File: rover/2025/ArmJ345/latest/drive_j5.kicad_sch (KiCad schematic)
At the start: 13 parts, among them J1 JST_PH_SB6, U1 IFX9201SGAUMA1, U2 CURR_SENSE-INA219AIDCNTG4

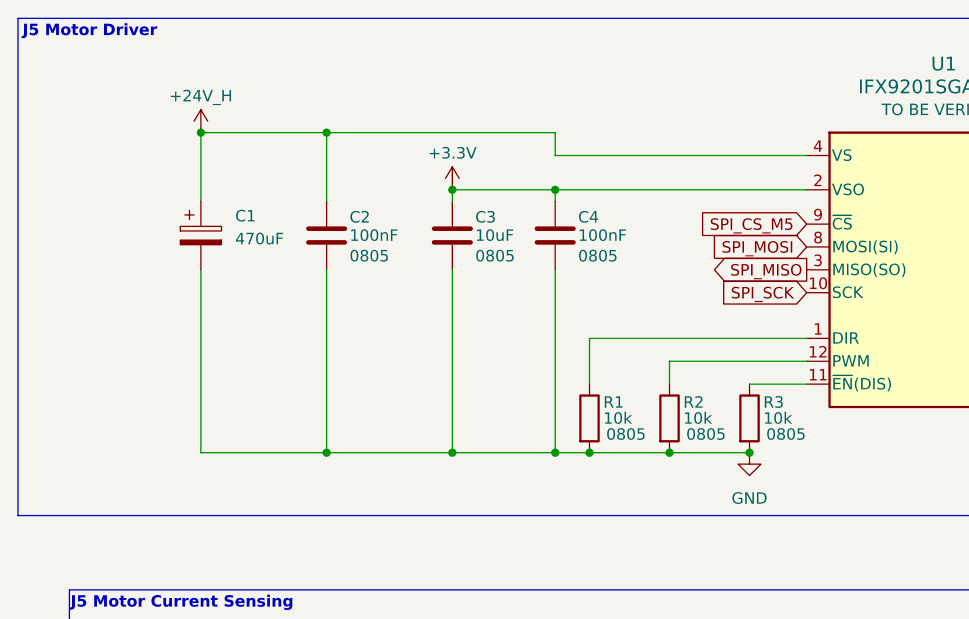
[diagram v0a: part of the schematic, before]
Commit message: armj345 fixes
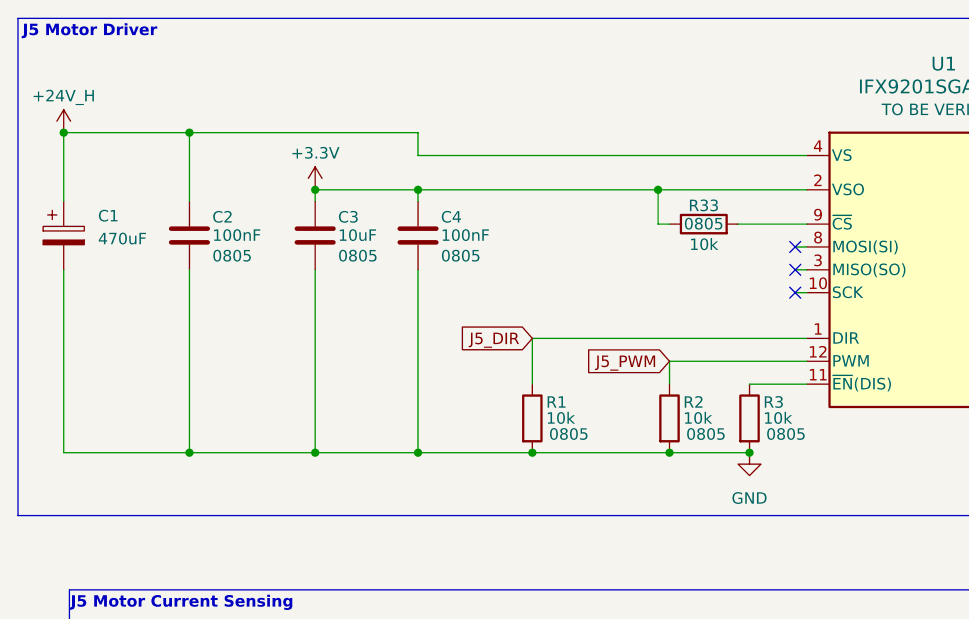
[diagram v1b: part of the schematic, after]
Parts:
- added R33: 10k, Resistor_SMD:R_0805_2012Metric_Pad1.20x1.40mm_HandSolder, symbol RoverLibrary:R_0805
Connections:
- net +3.3V: now also R33.1
- net J5_DIR: now reaches R1.1, U1.1 (DIR)
- net J5_PWM: now reaches R2.1, U1.12 (PWM)
- net SPI_CS_M5: no longer names the net of U1.9 (~{CS})
- net SPI_CS_M5: now also R33.2
- net SPI_MISO: no longer names the net of U1.3 (MISO(SO))
- net SPI_MOSI: no longer names the net of U1.8 (MOSI(SI))
- net SPI_SCK: no longer names the net of U1.10 (SCK)
- no-connect marks 1 -> 4
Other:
- moved on the sheet: C1, C2, C3, C4, R1

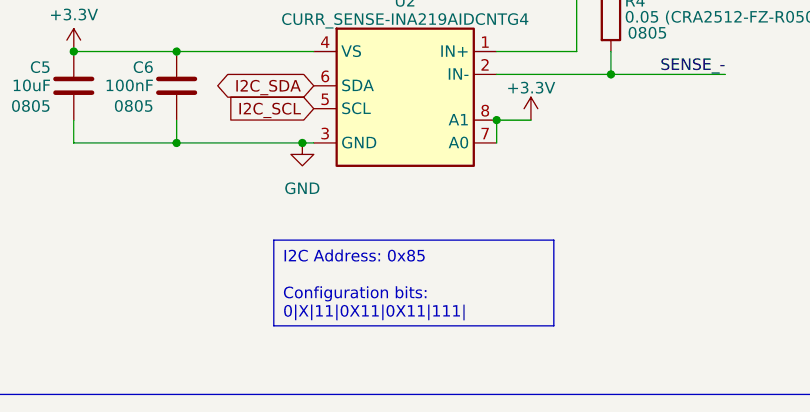
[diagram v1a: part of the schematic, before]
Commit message: Finished pcb layout for science module waiting on first review
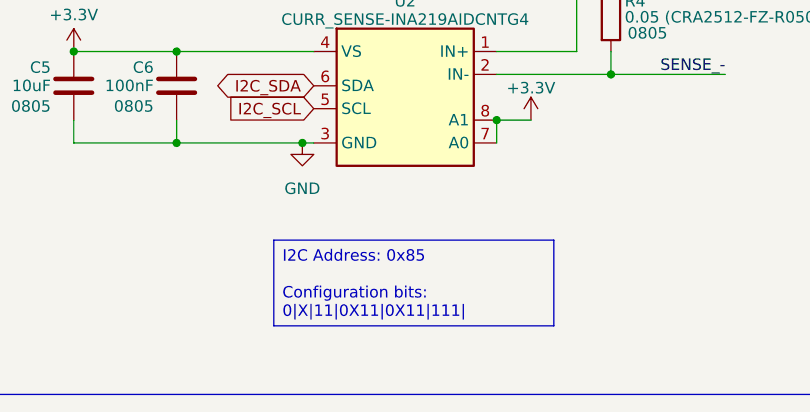
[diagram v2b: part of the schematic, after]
